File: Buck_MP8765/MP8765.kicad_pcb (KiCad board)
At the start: 2 copper layers, 40 x 20 mm, 28 parts, among them J1 Jumper

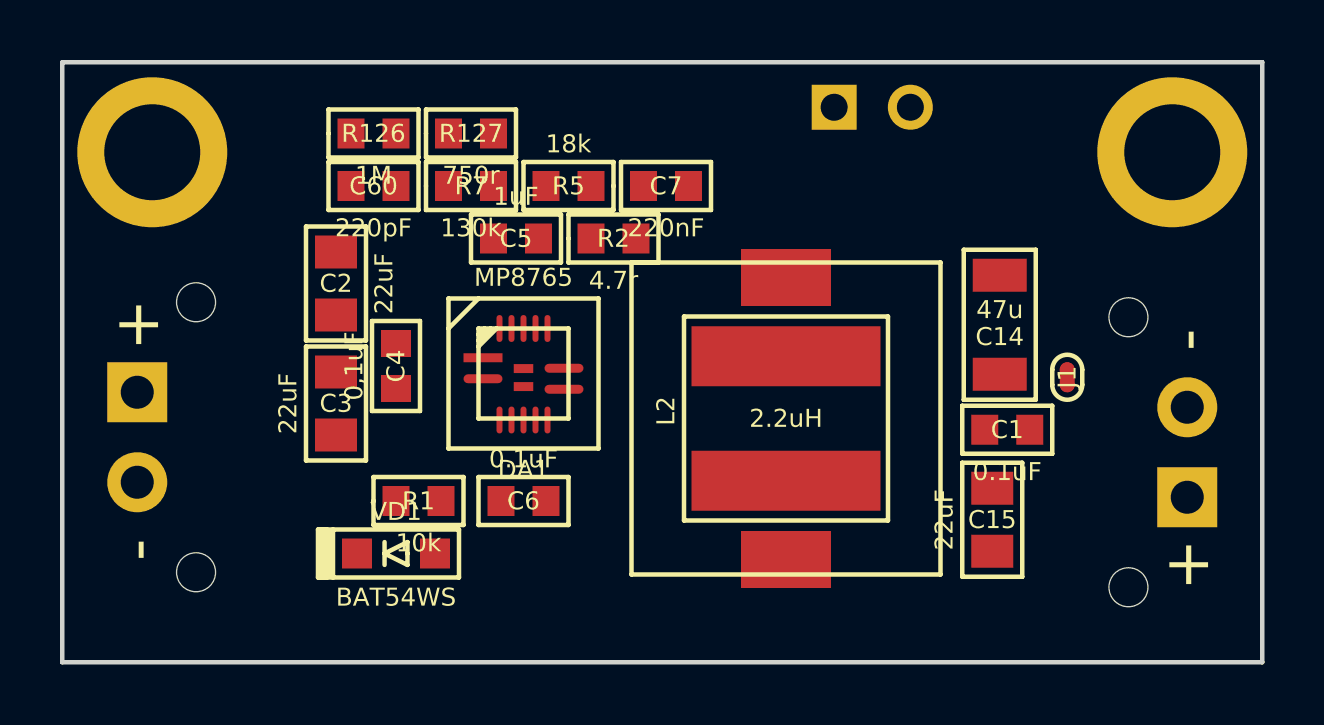
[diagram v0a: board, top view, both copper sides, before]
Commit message: ...
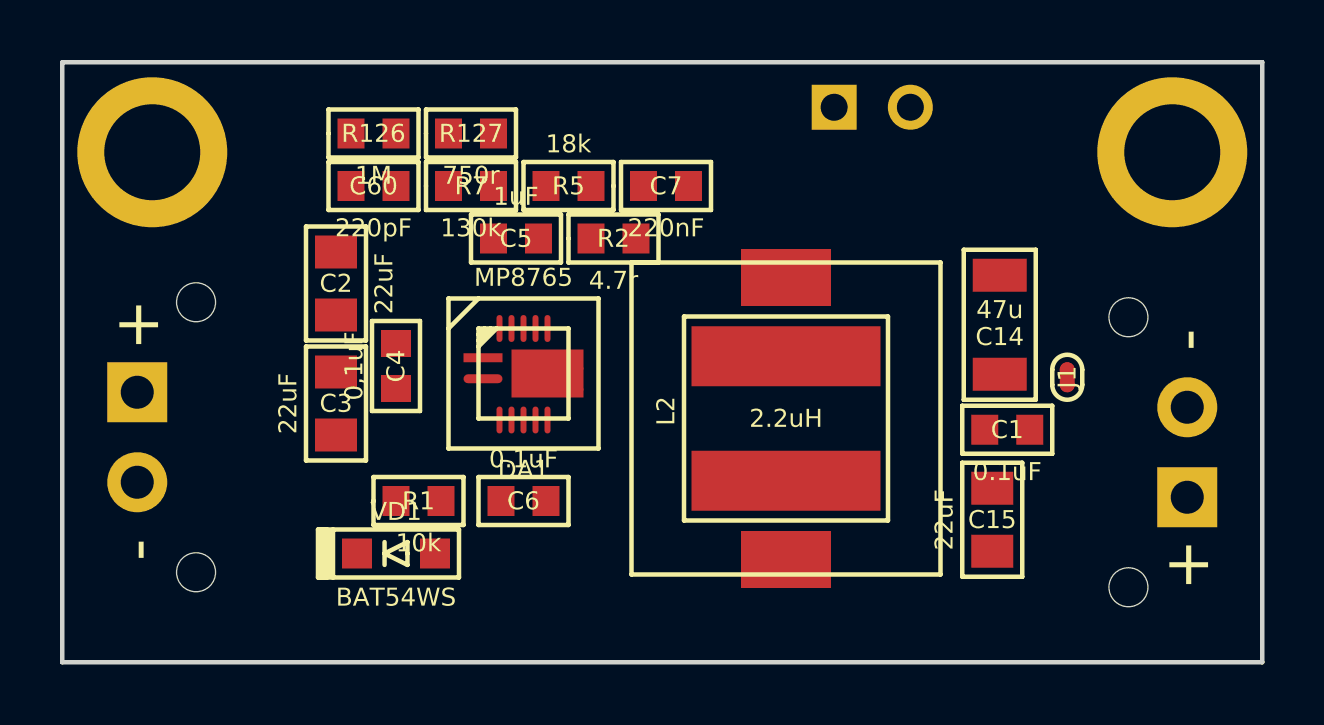
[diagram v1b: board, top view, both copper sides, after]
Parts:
- DA1: footprint QFN,_DFN,_LGA:FCQFN16 -> QFN,_DFN,_LGA:HFCQFN16
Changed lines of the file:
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@@
-(kicad_pcb (version 20171130) (host pcbnew "(5.0.0-rc2-dev-596-gcfd2f1d00)")
+(kicad_pcb (version 20171130) (host pcbnew "(5.1.5)-1")
   (general
     (thickness 1.6)
@@
     (zone_45_only no)
     (trace_min 0.2)
-    (segment_width 0.15)
-    (edge_width 0.15)
     (via_size 0.7)
     (via_drill 0.3)
@@
     (uvia_min_size 0.508)
     (uvia_min_drill 0.127)
+    (edge_width 0.15)
+    (segment_width 0.15)
     (pcb_text_width 0.3)
     (pcb_text_size 1.5 1.5)
@@
       (hpglpennumber 1)
       (hpglpenspeed 20)
-      (hpglpendiameter 15)
+      (hpglpendiameter 15.000000)
       (psnegative false)
       (psa4output false)
@@
       (drillshape 0)
       (scaleselection 1)
-      (outputdirectory Gerber/))
+      (outputdirectory "Gerber/"))
   )
   (net 0 "")
@@
     (uvia_dia 0.7)
     (uvia_drill 0.3)
+    (diff_pair_width 0.2)
     (diff_pair_gap 0.2)
-    (diff_pair_width 0.2)
     (add_net +5Vout)
     (add_net /5Vout_Good)
@@
     (uvia_dia 0.7)
     (uvia_drill 0.3)
+    (diff_pair_width 0.2)
     (diff_pair_gap 0.2)
-    (diff_pair_width 0.2)
     (add_net GND)
     (add_net GNDL1)
@@
     (uvia_dia 0.7)
     (uvia_drill 0.3)
+    (diff_pair_width 0.2)
     (diff_pair_gap 0.2)
-    (diff_pair_width 0.2)
   )
   (net_class wide1.0 ""
@@
     (uvia_dia 0.7)
     (uvia_drill 0.3)
+    (diff_pair_width 0.2)
     (diff_pair_gap 0.2)
-    (diff_pair_width 0.2)
   )
   (net_class wide1.5 ""
@@
     (uvia_dia 0.7)
     (uvia_drill 0.3)
+    (diff_pair_width 0.2)
     (diff_pair_gap 0.2)
-    (diff_pair_width 0.2)
     (add_net +12V)
     (add_net /+SW1)
@@
     (uvia_dia 0.7)
     (uvia_drill 0.3)
+    (diff_pair_width 0.2)
     (diff_pair_gap 0.2)
-    (diff_pair_width 0.2)
   )
   (net_class wide4.0 ""
@@
     (uvia_dia 0.7)
     (uvia_drill 0.3)
+    (diff_pair_width 0.2)
     (diff_pair_gap 0.2)
-    (diff_pair_width 0.2)
   )
   (module Capacitors:CAP0603 (layer F.Cu)
@@
       (rotate (xyz 0 0 0))
     )
-  )
-  (module QFN,_DFN,_LGA:FCQFN16 (layer F.Cu)
-    (at 115.375 60.375)
-    (attr smd)
-    (fp_text reference DA1 (at 0 3.2) (layer F.SilkS)
-      (effects (font (size 0.6 0.6) (thickness 0.15)))
-    )
-    (fp_text value MP8765 (at 0 -3.2) (layer F.SilkS)
-      (effects (font (size 0.6 0.6) (thickness 0.15)))
-    )
-    (fp_line (start -1.5 -1.5) (end 1.5 -1.5) (layer F.SilkS) (width 0.15))
-    (fp_line (start -1.5 1.5) (end -1.5 -1.5) (layer F.SilkS) (width 0.15))
-    (fp_line (start 1.5 1.5) (end -1.5 1.5) (layer F.SilkS) (width 0.15))
-    (fp_line (start 1.5 -1.5) (end 1.5 1.5) (layer F.SilkS) (width 0.15))
-    (fp_line (start -0.9 -1.5) (end -1.5 -0.9) (layer F.SilkS) (width 0.15))
-    (fp_line (start -2.5 2.5) (end -2.5 -2.5) (layer F.SilkS) (width 0.15))
-    (fp_line (start 2.5 2.5) (end -2.5 2.5) (layer F.SilkS) (width 0.15))
-    (fp_line (start 2.5 -2.5) (end 2.5 2.5) (layer F.SilkS) (width 0.15))
-    (fp_line (start -2.5 -2.5) (end 2.5 -2.5) (layer F.SilkS) (width 0.15))
-    (fp_line (start -1.5 -2.5) (end -2.5 -1.5) (layer F.SilkS) (width 0.15))
-    (fp_line (start -1.5 -1.3) (end -1.3 -1.5) (layer F.SilkS) (width 0.15))
-    (fp_line (start -1.5 -1.1) (end -1.1 -1.5) (layer F.SilkS) (width 0.15))
-    (pad 15 smd rect (at 0 -0.165) (size 0.65 0.3) (layers F.Cu F.Paste F.Mask))
-    (pad 16 smd rect (at 0 0.435) (size 0.65 0.3) (layers F.Cu F.Paste F.Mask))
-    (pad 9 smd oval (at 1.35 -0.175) (size 1.3 0.3) (layers F.Cu F.Paste F.Mask)
-      (net 5 /+SW1))
-    (pad 8 smd oval (at 1.35 0.525) (size 1.3 0.3) (layers F.Cu F.Paste F.Mask)
-      (net 5 /+SW1))
-    (pad 5 smd oval (at 0 1.55 270) (size 0.9 0.2) (layers F.Cu F.Paste F.Mask))
-    (pad 2 smd oval (at -1.35 0.175) (size 1.3 0.3) (layers F.Cu F.Paste F.Mask)
-      (net 1 GND))
-    (pad 1 smd rect (at -1.35 -0.525) (size 1.3 0.3) (layers F.Cu F.Paste F.Mask)
-      (net 2 +12V))
-    (pad 4 smd oval (at -0.4 1.55 270) (size 0.9 0.2) (layers F.Cu F.Paste F.Mask)
-      (net 8 /5Vout_Good))
-    (pad 3 smd oval (at -0.8 1.55 270) (size 0.9 0.2) (layers F.Cu F.Paste F.Mask))
-    (pad 6 smd oval (at 0.4 1.55 270) (size 0.9 0.2) (layers F.Cu F.Paste F.Mask)
-      (net 6 GNDL1))
-    (pad 7 smd oval (at 0.8 1.55 270) (size 0.9 0.2) (layers F.Cu F.Paste F.Mask)
-      (net 7 +5Vout))
-    (pad 10 smd oval (at 0.8 -1.5 270) (size 0.9 0.2) (layers F.Cu F.Paste F.Mask)
-      (net 10 "Net-(DA1-Pad10)"))
-    (pad 11 smd oval (at 0.4 -1.5 270) (size 0.9 0.2) (layers F.Cu F.Paste F.Mask)
-      (net 3 "Net-(C5-Pad1)"))
-    (pad 14 smd oval (at -0.8 -1.5 270) (size 0.9 0.2) (layers F.Cu F.Paste F.Mask)
-      (net 6 GNDL1))
-    (pad 13 smd oval (at -0.4 -1.5 270) (size 0.9 0.2) (layers F.Cu F.Paste F.Mask)
-      (net 12 /Enadle))
-    (pad 12 smd oval (at 0 -1.5 270) (size 0.9 0.2) (layers F.Cu F.Paste F.Mask)
-      (net 11 "Net-(DA1-Pad12)"))
   )
   (module "Installation:Heatsink_14x13(18)x6.2" (layer B.Cu)
@@
     (fp_circle (center 0.3 0) (end 0.2 0) (layer B.SilkS) (width 0.15))
   )
+  (module QFN,_DFN,_LGA:HFCQFN16 (layer F.Cu)
+    (at 115.375 60.375)
+    (attr smd)
+    (fp_text reference DA1 (at 0 3.2) (layer F.SilkS)
+      (effects (font (size 0.6 0.6) (thickness 0.15)))
+    )
+    (fp_text value MP8765 (at 0 -3.2) (layer F.SilkS)
+      (effects (font (size 0.6 0.6) (thickness 0.15)))
+    )
+    (fp_line (start -1.5 -1.5) (end 1.5 -1.5) (layer F.SilkS) (width 0.15))
+    (fp_line (start -1.5 1.5) (end -1.5 -1.5) (layer F.SilkS) (width 0.15))
+    (fp_line (start 1.5 1.5) (end -1.5 1.5) (layer F.SilkS) (width 0.15))
+    (fp_line (start 1.5 -1.5) (end 1.5 1.5) (layer F.SilkS) (width 0.15))
+    (fp_line (start -0.9 -1.5) (end -1.5 -0.9) (layer F.SilkS) (width 0.15))
+    (fp_line (start -2.5 2.5) (end -2.5 -2.5) (layer F.SilkS) (width 0.15))
+    (fp_line (start 2.5 2.5) (end -2.5 2.5) (layer F.SilkS) (width 0.15))
+    (fp_line (start 2.5 -2.5) (end 2.5 2.5) (layer F.SilkS) (width 0.15))
+    (fp_line (start -2.5 -2.5) (end 2.5 -2.5) (layer F.SilkS) (width 0.15))
+    (fp_line (start -1.5 -2.5) (end -2.5 -1.5) (layer F.SilkS) (width 0.15))
+    (fp_line (start -1.5 -1.3) (end -1.3 -1.5) (layer F.SilkS) (width 0.15))
+    (fp_line (start -1.5 -1.1) (end -1.1 -1.5) (layer F.SilkS) (width 0.15))
+    (pad 15 smd rect (at 0 -0.165) (size 0.65 0.3) (layers F.Cu F.Paste F.Mask))
+    (pad 16 smd rect (at 0 0.435) (size 0.65 0.3) (layers F.Cu F.Paste F.Mask))
+    (pad 9 smd oval (at 1.35 -0.175) (size 1.3 0.3) (layers F.Cu F.Paste F.Mask)
+      (net 5 /+SW1))
+    (pad 8 smd oval (at 1.35 0.525) (size 1.3 0.3) (layers F.Cu F.Paste F.Mask)
+      (net 5 /+SW1))
+    (pad 5 smd oval (at 0 1.55 270) (size 0.9 0.2) (layers F.Cu F.Paste F.Mask))
+    (pad 2 smd oval (at -1.35 0.175) (size 1.3 0.3) (layers F.Cu F.Paste F.Mask)
+      (net 1 GND))
+    (pad 1 smd rect (at -1.35 -0.525) (size 1.3 0.3) (layers F.Cu F.Paste F.Mask)
+      (net 2 +12V))
+    (pad 4 smd oval (at -0.4 1.55 270) (size 0.9 0.2) (layers F.Cu F.Paste F.Mask)
+      (net 8 /5Vout_Good))
+    (pad 3 smd oval (at -0.8 1.55 270) (size 0.9 0.2) (layers F.Cu F.Paste F.Mask))
+    (pad 6 smd oval (at 0.4 1.55 270) (size 0.9 0.2) (layers F.Cu F.Paste F.Mask)
+      (net 6 GNDL1))
+    (pad 7 smd oval (at 0.8 1.55 270) (size 0.9 0.2) (layers F.Cu F.Paste F.Mask)
+      (net 7 +5Vout))
+    (pad 10 smd oval (at 0.8 -1.5 270) (size 0.9 0.2) (layers F.Cu F.Paste F.Mask)
+      (net 10 "Net-(DA1-Pad10)"))
+    (pad 11 smd oval (at 0.4 -1.5 270) (size 0.9 0.2) (layers F.Cu F.Paste F.Mask)
+      (net 3 "Net-(C5-Pad1)"))
+    (pad 14 smd oval (at -0.8 -1.5 270) (size 0.9 0.2) (layers F.Cu F.Paste F.Mask)
+      (net 6 GNDL1))
+    (pad 13 smd oval (at -0.4 -1.5 270) (size 0.9 0.2) (layers F.Cu F.Paste F.Mask)
+      (net 12 /Enadle))
+    (pad 12 smd oval (at 0 -1.5 270) (size 0.9 0.2) (layers F.Cu F.Paste F.Mask)
+      (net 11 "Net-(DA1-Pad12)"))
+    (pad 9 smd rect (at 0.8 0) (size 2.4 1.6) (layers F.Cu)
+      (net 5 /+SW1))
+  )
   (gr_line (start 100 70) (end 100 50) (angle 90) (layer Edge.Cuts) (width 0.15))
